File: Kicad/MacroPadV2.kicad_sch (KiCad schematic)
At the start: 31 parts, among them K1 KSW, K10 KSW, K11 KSW, K12 KSW, K2 KSW, K3 KSW, K4 KSW, K5 KSW, K6 KSW, K7 KSW, K8 KSW, K9 KSW, SW1 RotaryEncoder_Switch, U1 SparkFunProMicro

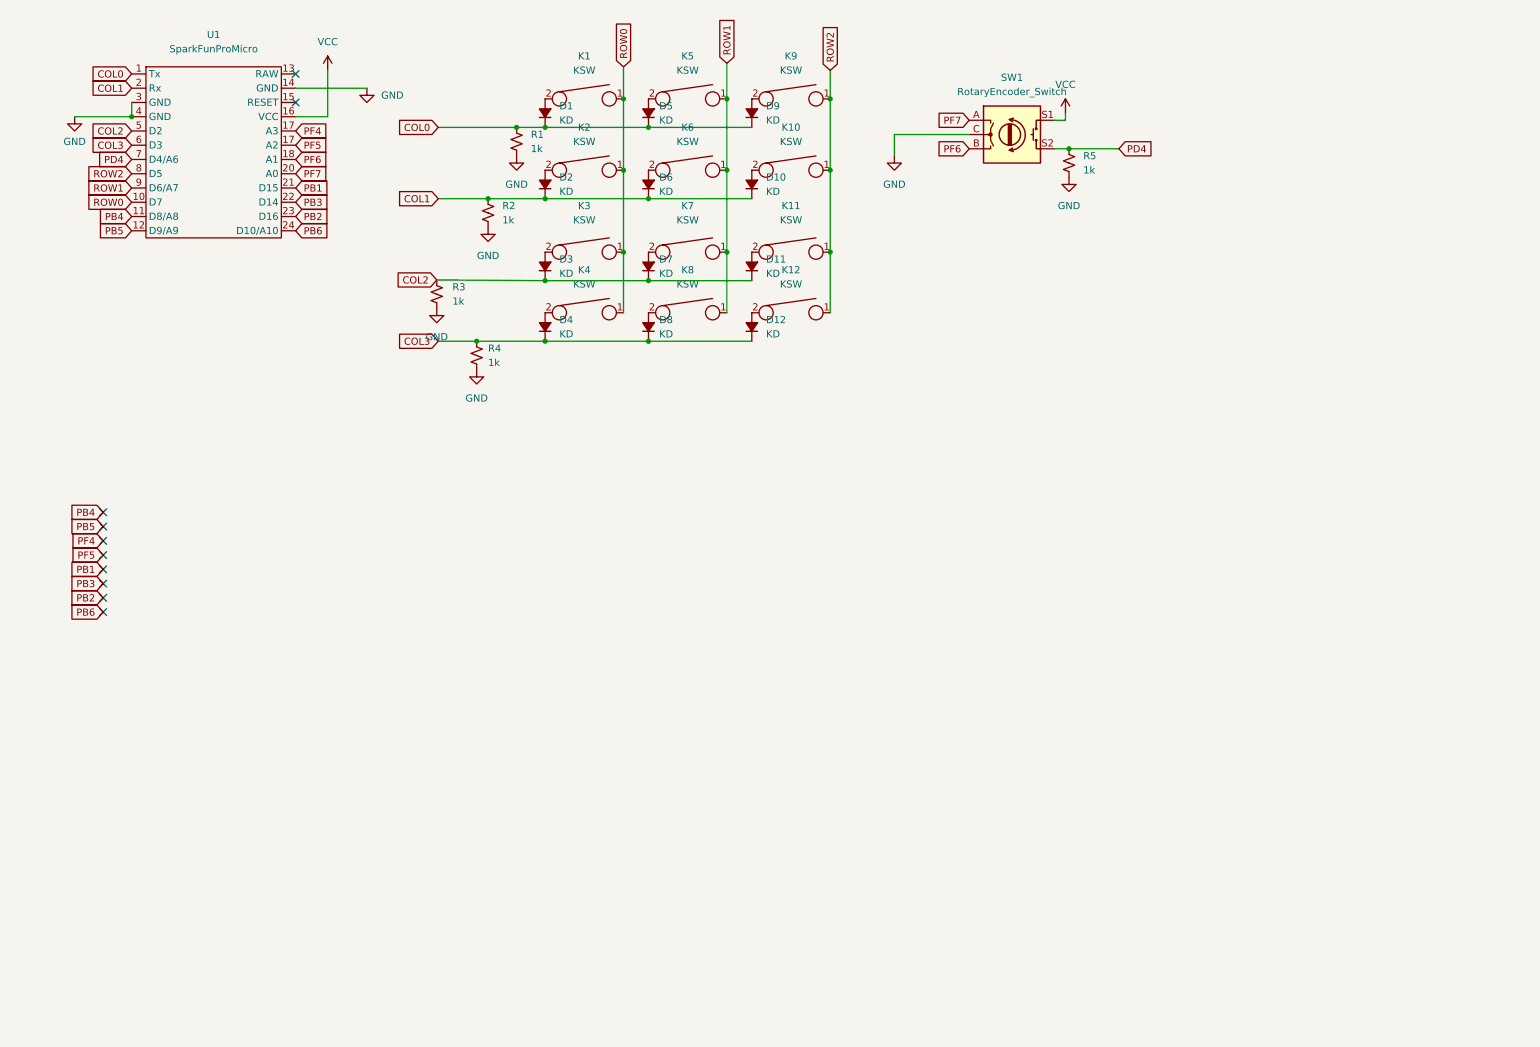
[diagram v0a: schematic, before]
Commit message: New LAyout an Routing done
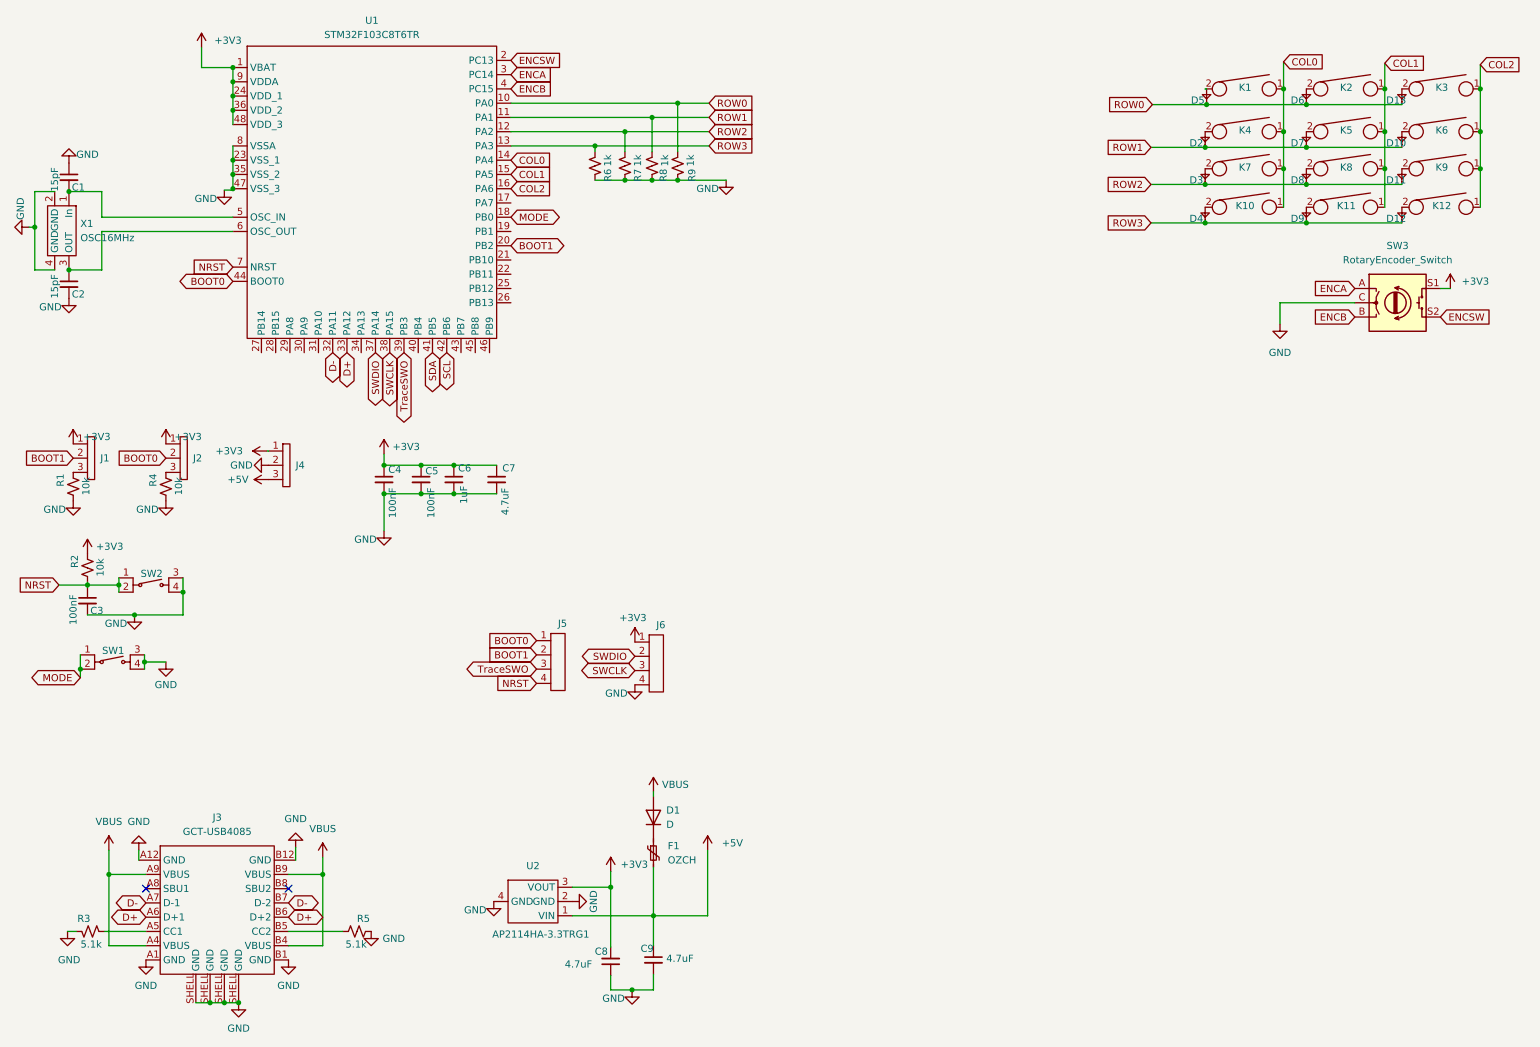
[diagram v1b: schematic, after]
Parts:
- removed D1, D10, D11, D12, D2, D3, D4, D5, D6, D7, D8, D9: KD, mpadfps:sod323, symbol Device:D_Small_Filled
- removed U1: SparkFunProMicro, aarohanl:SparkFrunProMicro, symbol macropad_parts:SparkFunProMicro
- added C1, C2: 15pF, Capacitor_SMD:C_0805_2012Metric_Pad1.18x1.45mm_HandSolder, symbol Device:C_Small
- added C3, C4, C5: 100nF, Capacitor_SMD:C_0805_2012Metric_Pad1.18x1.45mm_HandSolder, symbol Device:C_Small
- added C6: 1uF, Capacitor_SMD:C_0805_2012Metric_Pad1.18x1.45mm_HandSolder, symbol Device:C_Small
- added C7, C8, C9: 4.7uF, Capacitor_SMD:C_0805_2012Metric_Pad1.18x1.45mm_HandSolder, symbol Device:C_Small
- added D1: D, Diode_SMD:D_0805_2012Metric_Pad1.15x1.40mm_HandSolder, symbol Device:D
- added D10, D11, D12, D13, D2, D3, D4, D5, D6, D7, D8, D9: 1N4148WX-TP, Diode_SMD:D_0805_2012Metric_Pad1.15x1.40mm_HandSolder, symbol symbols:1N4148WX-TP
- added F1: OZCH, mpadfps:OZCHFusr, symbol Device:Polyfuse_Small
- added J1, J2, J4: 3PinJump, Connector_PinHeader_2.54mm:PinHeader_1x03_P2.54mm_Vertical, symbol macropad_parts:3PinJump
- added J3: GCT-USB4085, mpadfps:USB4085-GF-A, symbol symbols:GCT-USB4085
- added J5, J6: 4PinJump, Connector_PinHeader_2.54mm:PinHeader_1x04_P2.54mm_Vertical, symbol macropad_parts:4PinJump
- added R6, R7, R8, R9: 1k, Resistor_SMD:R_0805_2012Metric_Pad1.20x1.40mm_HandSolder, symbol Device:R_Small_US
- added SW1, SW2: SWITCH_TACTILE_SPST-NO_0.05A_12V, mpadfps:PTS645-G, symbol macropad_parts:SWITCH_TACTILE_SPST-NO_0.05A_12V
- added U1: STM32F103C8T6TR, mpadfps:LQFP48, symbol symbols:STM32F103C8T6TR
- added U2: AP2114HA-3.3TRG1, keyboard_fp:SOT-223_DIO-L, symbol macropad_parts:AP2114HA-3.3TRG1
- added X1: TSX-3225_16.0000MF18X-AC6, mpadfps:TSX-3226, symbol macropad_parts:TSX-3225_16.0000MF18X-AC6
- K1, K10, K11, K12, K2, K3, K4, K5, K6, K7, K8, K9: footprint aarohanl:CherryMxFP -> keyboard_fp:CherryMx
- R1, R2, R4: value 1k -> 10k
- R3, R5: value 1k -> 5.1k
- SW3: renamed from SW1; footprint aarohanl:PEC11H4020FS0016_PinCorrection -> mpadfps:PEC11H-RotaryEncoderSwitch
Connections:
- net COL0: now also K1.1, K10.1, K4.1, K7.1, U1.14 (PA4); no longer R1.1
- net COL1: now also K11.1, K2.1, K5.1, K8.1, U1.15 (PA5); no longer R2.1
- net COL2: now also K12.1, K3.1, K6.1, K9.1, U1.16 (PA6); no longer R3.1
- net GND: now also R3.1, R5.1, C1.1, C2.2, C3.2, C4.2, C5.2, C6.2, C7.2, C8.1, C9.2, J3.A1 (GND), J3.A12 (GND), J3.B1 (GND), J3.B12 (GND), J3.SHELL (GND), J4.2, J6.4, R6.1, R7.1, R8.1, R9.1, SW1.3, SW1.4, SW2.3, SW2.4, U1.23 (VSS_1), U1.35 (VSS_2), U1.47 (VSS_3), U1.8 (VSSA), U2.2 (GND), U2.4 (GND), X1.2 (GND), X1.4 (GND); no longer R2.2, R3.2, R5.2
- net ROW0: now also D13.2, D5.2, D6.2, R9.2, U1.10 (PA0); no longer K1.1, K2.1, K3.1, K4.1
- net ROW1: now also D10.2, D2.2, D7.2, R8.2, U1.11 (PA1); no longer K5.1, K6.1, K7.1, K8.1
- net ROW2: now also D11.2, D3.2, D8.2, R7.2, U1.12 (PA2); no longer K10.1, K11.1, K12.1, K9.1
- net at K8.2: now also D8.1
- net at K5.2: now also D7.1
- net at K2.2: now also D6.1
- net at K10.2: now also D4.1
- net at K12.2: now also D12.1
- net at K6.2: now also D10.1
- net at K4.2: now also D2.1
- net at K1.2: now also D5.1
- net at K7.2: now also D3.1
- net at K9.2: now also D11.1
- net at K11.2: now also D9.1
- net at K3.2: now also D13.1
- net COL3: no longer names the net of R4.1
- net COL3: now also J2.3
- net PD4 renamed ENCSW
- net ENCSW: now also U1.2 (PC13); no longer R5.1
- net PF6 renamed ENCB
- net ENCB: now also U1.4 (PC15)
- net PF7 renamed ENCA
- net ENCA: now also U1.3 (PC14)
- net VCC renamed +3V3
- net +3V3: now also R2.1, C4.1, C5.1, C6.1, C7.1, C8.2, J1.1, J2.1, J4.1, J6.1, U1.1 (VBAT), U1.24 (VDD_1), U1.36 (VDD_2), U1.48 (VDD_3), U1.9 (VDDA), U2.3 (VOUT)
- new net: C1.2, U1.5 (OSC_IN), X1.1 (In)
- new net: J3.B5 (CC2), R5.2
- new net: J3.A5 (CC1), R3.2
- new net: C2.1, U1.6 (OSC_OUT), X1.3 (OUT)
- new net: D1.1 (K), F1.1
- new net: J1.3, R1.1
- new net +5V: C9.1, F1.2, J4.3, U2.1 (VIN)
- new net BOOT0: J2.2, J5.1, U1.44 (BOOT0)
- new net BOOT1: J1.2, J5.2, U1.20 (PB2)
- new net D+: J3.A6 (D+1), J3.B6 (D+2), U1.33 (PA12)
- new net D-: J3.A7 (D-1), J3.B7 (D-2), U1.32 (PA11)
- new net MODE: SW1.1, SW1.2, U1.18 (PB0)
- new net NRST: C3.1, J5.4, R2.2, SW2.1, SW2.2, U1.7 (NRST)
- new net ROW3: D12.2, D4.2, D9.2, R6.2, U1.13 (PA3)
- new net SCL: U1.42 (PB6)
- new net SDA: U1.41 (PB5)
- new net SWCLK: J6.3, U1.38 (PA15)
- new net SWDIO: J6.2, U1.37 (PA14)
- new net TraceSWO: J5.3, U1.39 (PB3)
- new net VBUS: D1.2 (A), J3.A4 (VBUS), J3.A9 (VBUS), J3.B4 (VBUS), J3.B9 (VBUS)
- no-connect marks 10 -> 2
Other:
- moved on the sheet: K1, SW3
